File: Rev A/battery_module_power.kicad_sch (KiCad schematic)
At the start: 17 parts, among them Q1 IRLZ44N, Q2 BC337, Q4 BC337, Q5 BC327

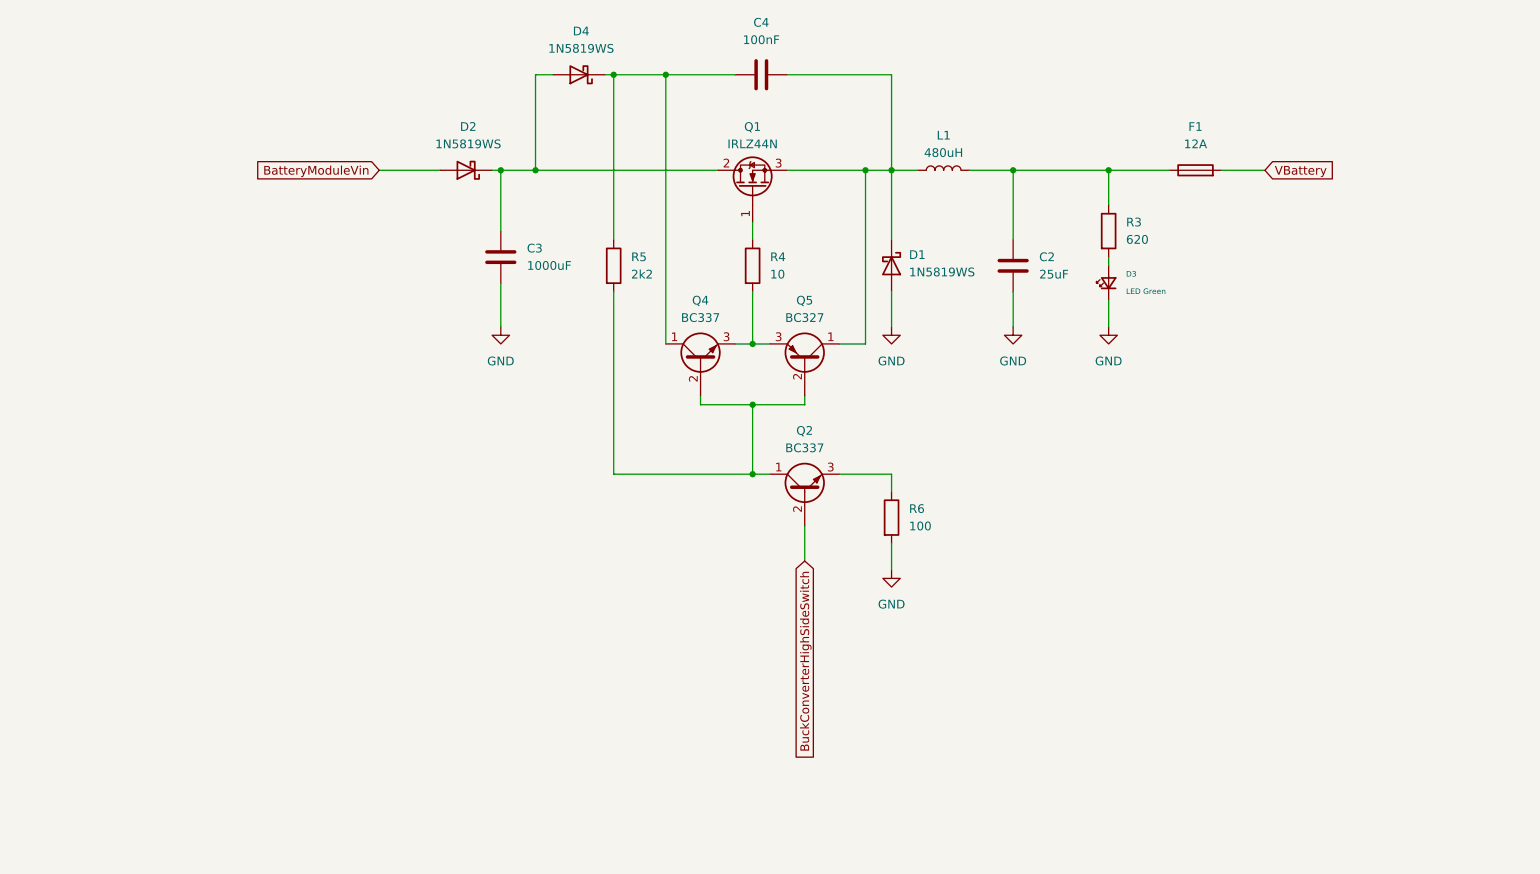
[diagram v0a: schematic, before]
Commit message: Updated buck.
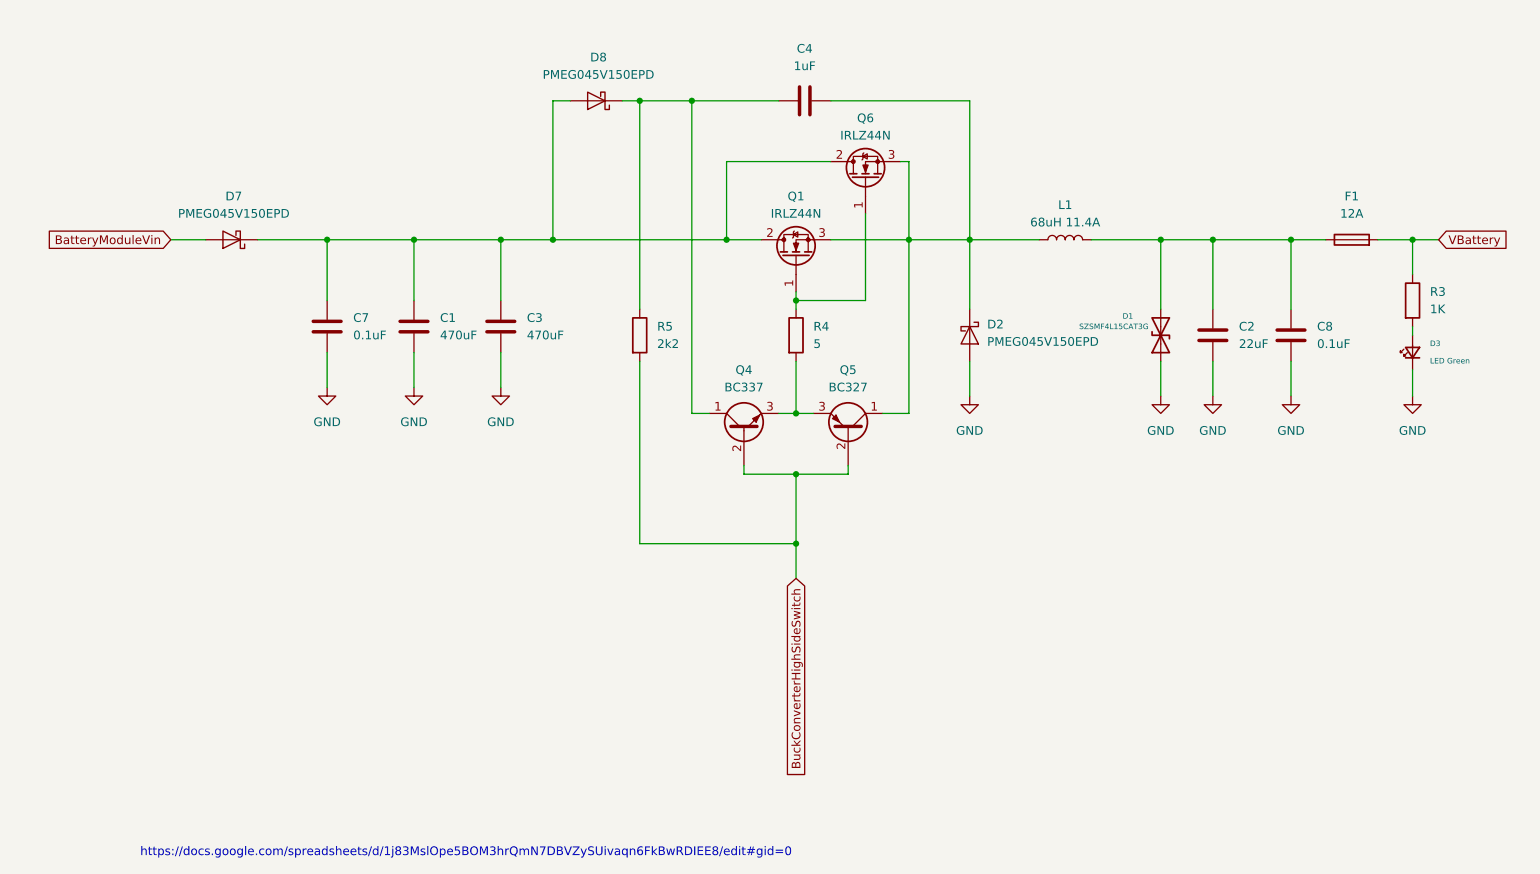
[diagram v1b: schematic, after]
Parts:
- removed D1, D2, D4: 1N5819WS, Diode_SMD:D_SOD-323, symbol Diode:1N5819WS
- removed Q2: BC337, Package_TO_SOT_THT:TO-92_Inline, symbol Transistor_BJT:BC337
- removed R6: 100, symbol Device:R
- added C1: 470uF, symbol Device:C
- added C7, C8: 0.1uF, Capacitor_SMD:C_0805_2012Metric, symbol Device:C
- added D1: SZSMF4L15CAT3G, Diode_SMD:D_SOD-123F, symbol Device:D_TVS
- added D2, D7, D8: PMEG045V150EPD, Package_TO_SOT_SMD:Nexperia_CFP15_SOT-1289, symbol Diode:PMEG045V150EPD
- added Q6: IRLZ44N, Package_TO_SOT_THT:TO-220-3_Vertical, symbol Transistor_FET:IRLZ44N
- C2: value 25uF -> 22uF
- C3: value 1000uF -> 470uF
- C4: value 100nF -> 1uF; footprint (none) -> Capacitor_SMD:C_0805_2012Metric
- L1: value 480uH -> 68uH 11.4A
- R3: value 620 -> 1K; footprint (none) -> Resistor_SMD:R_0805_2012Metric
- R4: value 10 -> 5; footprint (none) -> Resistor_SMD:R_0805_2012Metric
- R5: footprint (none) -> Resistor_SMD:R_0805_2012Metric
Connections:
- net BatteryModuleVin: now also D7.1 (A), D7.2 (A)
- net BuckConverterHighSideSwitch: now also Q4.2 (B), Q5.2 (B), R5.2
- net GND: now also C1.2, C7.2, C8.2, D1.1 (A1), D2.1 (A), D2.2 (A)
- net VBattery: now also R3.1
- net at C2.1, F1.1, L1.2: now also C8.1, D1.2 (A2); no longer R3.1
- net at C4.1, Q4.1 (C), R5.1: now also D8.3 (K)
- net at C3.1, Q1.2 (D): now also C1.1, C7.1, D7.3 (K), D8.1 (A), D8.2 (A), Q6.2 (D)
- net at C4.2, L1.1, Q1.3 (S)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: now also D2.3 (K), Q6.3 (S)
- net at Q1.1 (G), R4.1: now also Q6.1 (G)
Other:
- note added: "https://docs.google.com/spreadsheets/d/1j83MslOpe5BOM3hrQmN7DBVZySUivaqn6FkBwRDIEE8/edit#gid=0"
- moved on the sheet: C2, C3, C4, D3, F1, L1, Q1, Q4, Q5, R3, R4, R5
